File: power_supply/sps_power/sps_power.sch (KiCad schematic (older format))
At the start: 10 parts, among them U1 MC33063AD

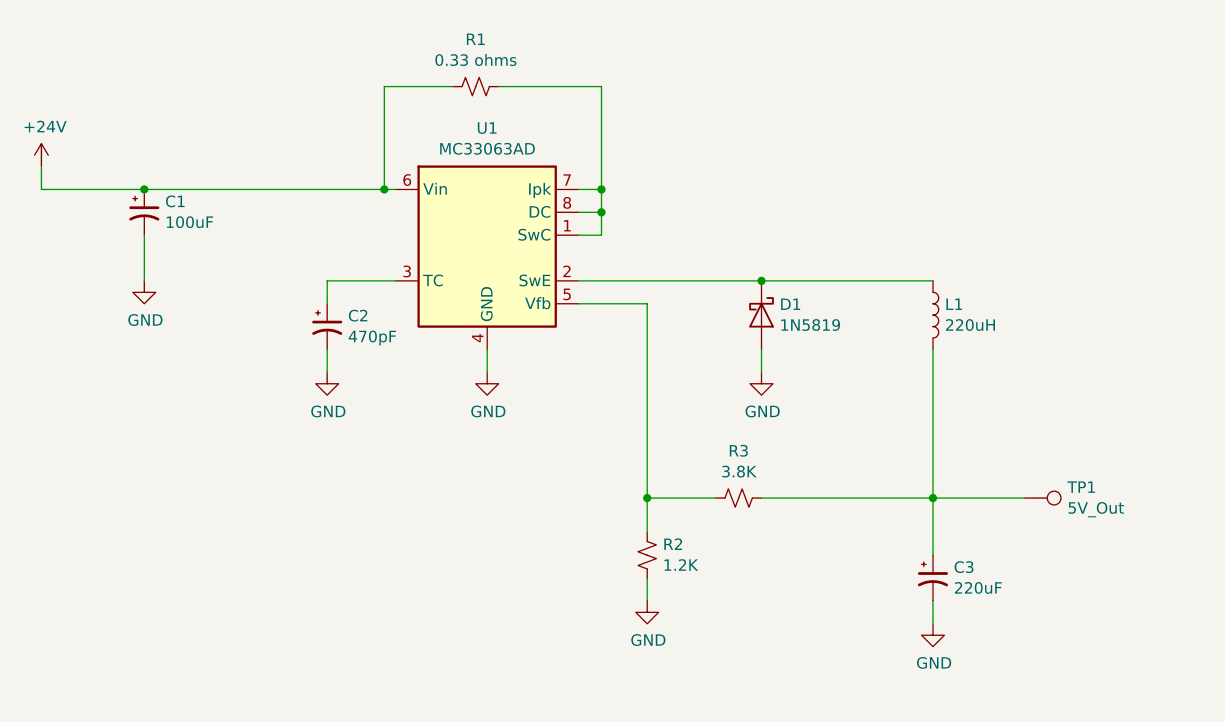
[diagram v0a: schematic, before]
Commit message: Interum power supply cad commit
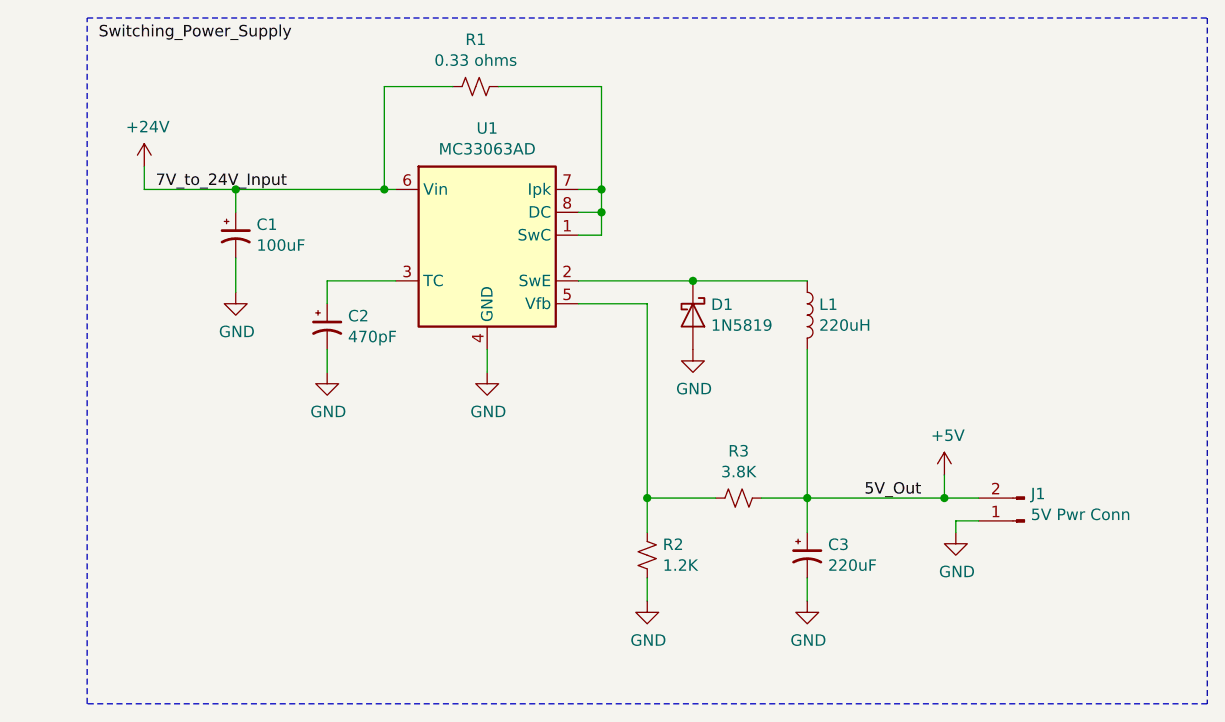
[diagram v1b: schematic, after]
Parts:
- removed TP1: 5V_Out, TestPoint:TestPoint_Pad_D2.0mm, symbol Connector:TestPoint
- added J1: 5V Pwr Conn, Connector_PinHeader_1.00mm:PinHeader_1x02_P1.00mm_Vertical, symbol Connector:Conn_01x02_Male
- U1: Supplier (none) -> DigiKey; Supplier Part (none) -> 296-17763-1-ND
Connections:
- net GND: now also J1.1 (Pin_1)
- net +5V: now reaches C3.1, L1.2, R3.2
- net +5V: now also J1.2 (Pin_2)
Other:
- moved on the sheet: C1, C3, D1, L1
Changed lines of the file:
@@
 $EndDescr
-$Comp
-L Regulator_Switching:MC33063AD U1
-U 1 1 5E7FFA3D
-P 4850 3550
-F 0 "U1" H 4850 4017 50  0000 C CNN
-F 1 "MC33063AD" H 4850 3926 50  0000 C CNN
-F 2 "Package_SO:SOIC-8_3.9x4.9mm_P1.27mm" H 4900 3100 50  0001 L CNN
-F 3 "http://www.onsemi.com/pub_link/Collateral/MC34063A-D.PDF" H 5350 3450 50  0001 C CNN
-	1    4850 3550
-	1    0    0    -1
-$EndComp
 $Comp
 L power:GND #PWR0101
@@
 L Device:CP1_Small C3
 U 1 1 5E805CD8
-P 6800 5050
-F 0 "C3" H 6891 5096 50  0000 L CNN
-F 1 "220uF" H 6891 5005 50  0000 L CNN
-F 2 "Capacitor_SMD:CP_Elec_10x10" H 6800 5050 50  0001 C CNN
-F 3 "~" H 6800 5050 50  0001 C CNN
-F 4 "493-6277-1-ND" H 6800 5050 50  0001 C CNN "Supplier Part"
-F 5 "Digikey" H 6800 5050 50  0001 C CNN "Supplier"
-	1    6800 5050
+P 6250 4950
+F 0 "C3" H 6341 4996 50  0000 L CNN
+F 1 "220uF" H 6341 4905 50  0000 L CNN
+F 2 "Capacitor_SMD:CP_Elec_10x10" H 6250 4950 50  0001 C CNN
+F 3 "~" H 6250 4950 50  0001 C CNN
+F 4 "493-6277-1-ND" H 6250 4950 50  0001 C CNN "Supplier Part"
+F 5 "Digikey" H 6250 4950 50  0001 C CNN "Supplier"
+	1    6250 4950
 	1    0    0    -1
 $EndComp
@@
 L Device:D_Schottky D1
 U 1 1 5E806E01
-P 6050 3900
-F 0 "D1" V 6004 3979 50  0000 L CNN
-F 1 "1N5819" V 6095 3979 50  0000 L CNN
-F 2 "Diode_SMD:D_SOD-123" H 6050 3900 50  0001 C CNN
-F 3 "~" H 6050 3900 50  0001 C CNN
-F 4 "DigiKey" V 6050 3900 50  0001 C CNN "Supplier"
-F 5 "1N5819HW-FDIDKR-ND" V 6050 3900 50  0001 C CNN "Supplier Part"
-	1    6050 3900
+P 5750 3900
+F 0 "D1" V 5704 3979 50  0000 L CNN
+F 1 "1N5819" V 5795 3979 50  0000 L CNN
+F 2 "Diode_SMD:D_SOD-123" H 5750 3900 50  0001 C CNN
+F 3 "~" H 5750 3900 50  0001 C CNN
+F 4 "DigiKey" V 5750 3900 50  0001 C CNN "Supplier"
+F 5 "1N5819HW-FDIDKR-ND" V 5750 3900 50  0001 C CNN "Supplier Part"
+	1    5750 3900
 	0    1    1    0
-$EndComp
-$Comp
-L Device:CP1_Small C1
-U 1 1 5E810EBD
-P 3350 3450
-F 0 "C1" H 3441 3496 50  0000 L CNN
-F 1 "100uF" H 3441 3405 50  0000 L CNN
-F 2 "Capacitor_THT:CP_Radial_D5.0mm_P2.50mm" H 3350 3450 50  0001 C CNN
-F 3 "~" H 3350 3450 50  0001 C CNN
-F 4 "493-2203-1-ND" H 3350 3450 50  0001 C CNN "Supplier Part"
-F 5 "Digikey" H 3350 3450 50  0001 C CNN "Supplier"
-	1    3350 3450
-	1    0    0    -1
 $EndComp
 $Comp
 L power:GND #PWR0103
 U 1 1 5E81AA34
-P 3350 3750
-F 0 "#PWR0103" H 3350 3500 50  0001 C CNN
-F 1 "GND" H 3355 3577 50  0000 C CNN
-F 2 "" H 3350 3750 50  0001 C CNN
-F 3 "" H 3350 3750 50  0001 C CNN
-	1    3350 3750
-	1    0    0    -1
-$EndComp
-Wire Wire Line
-	3350 3550 3350 3750
+P 3750 3800
+F 0 "#PWR0103" H 3750 3550 50  0001 C CNN
+F 1 "GND" H 3755 3627 50  0000 C CNN
+F 2 "" H 3750 3800 50  0001 C CNN
+F 3 "" H 3750 3800 50  0001 C CNN
+	1    3750 3800
+	1    0    0    -1
+$EndComp
 $Comp
 L Device:R_Small_US R3
@@
 	5250 3350 5350 3350
 Wire Wire Line
-	2900 3250 2900 3350
-Wire Wire Line
-	2900 3350 3350 3350
-Connection ~ 3350 3350
-Wire Wire Line
-	3350 3350 4400 3350
-Wire Wire Line
 	4450 3350 4400 3350
 Connection ~ 4400 3350
@@
 Connection ~ 5350 3450
 Wire Wire Line
-	5250 3750 6050 3750
+	5250 3750 5750 3750
 $Comp
 L Device:L L1
 U 1 1 5E801D9A
-P 6800 3900
-F 0 "L1" H 6852 3946 50  0000 L CNN
-F 1 "220uH" H 6852 3855 50  0000 L CNN
-F 2 "Inductor_SMD:L_Bourns-SRR1005" H 6800 3900 50  0001 C CNN
-F 3 "~" H 6800 3900 50  0001 C CNN
-F 4 "Digikey" H 6800 3900 50  0001 C CNN "Supplier"
-F 5 "SDR1806-221KLCT-ND" H 6800 3900 50  0001 C CNN "Supplier Part"
-	1    6800 3900
-	1    0    0    -1
-$EndComp
-Wire Wire Line
-	6050 3750 6800 3750
-Connection ~ 6050 3750
+P 6250 3900
+F 0 "L1" H 6302 3946 50  0000 L CNN
+F 1 "220uH" H 6302 3855 50  0000 L CNN
+F 2 "Inductor_SMD:L_Bourns-SRR1005" H 6250 3900 50  0001 C CNN
+F 3 "~" H 6250 3900 50  0001 C CNN
+F 4 "Digikey" H 6250 3900 50  0001 C CNN "Supplier"
+F 5 "SDR1806-221KLCT-ND" H 6250 3900 50  0001 C CNN "Supplier Part"
+	1    6250 3900
+	1    0    0    -1
+$EndComp
 Wire Wire Line
 	4850 4050 4850 4150
@@
 L power:GND #PWR0105
 U 1 1 5E863A3A
-P 6800 5250
-F 0 "#PWR0105" H 6800 5000 50  0001 C CNN
-F 1 "GND" H 6805 5077 50  0000 C CNN
-F 2 "" H 6800 5250 50  0001 C CNN
-F 3 "" H 6800 5250 50  0001 C CNN
-	1    6800 5250
-	1    0    0    -1
-$EndComp
-Wire Wire Line
-	6800 5150 6800 5250
-Wire Wire Line
-	6800 4050 6800 4700
+P 6250 5150
+F 0 "#PWR0105" H 6250 4900 50  0001 C CNN
+F 1 "GND" H 6255 4977 50  0000 C CNN
+F 2 "" H 6250 5150 50  0001 C CNN
+F 3 "" H 6250 5150 50  0001 C CNN
+	1    6250 5150
+	1    0    0    -1
+$EndComp
 Wire Wire Line
 	5250 3850 5550 3850
@@
 Connection ~ 5550 4700
 Wire Wire Line
-	6050 4700 6800 4700
-Connection ~ 6800 4700
-Wire Wire Line
-	6800 4700 6800 4950
-$Comp
-L Connector:TestPoint TP1
-U 1 1 5E86A93E
-P 7200 4700
-F 0 "TP1" V 7154 4888 50  0000 L CNN
-F 1 "5V_Out" V 7245 4888 50  0000 L CNN
-F 2 "TestPoint:TestPoint_Pad_D2.0mm" H 7400 4700 50  0001 C CNN
-F 3 "~" H 7400 4700 50  0001 C CNN
-	1    7200 4700
-	0    1    1    0
-$EndComp
-Wire Wire Line
-	6800 4700 7200 4700
+	6050 4700 6250 4700
 $Comp
 L power:GND #PWR0106
 U 1 1 5E86CC9B
-P 6050 4150
-F 0 "#PWR0106" H 6050 3900 50  0001 C CNN
-F 1 "GND" H 6055 3977 50  0000 C CNN
-F 2 "" H 6050 4150 50  0001 C CNN
-F 3 "" H 6050 4150 50  0001 C CNN
-	1    6050 4150
-	1    0    0    -1
-$EndComp
-Wire Wire Line
-	6050 4050 6050 4150
+P 5750 4050
+F 0 "#PWR0106" H 5750 3800 50  0001 C CNN
+F 1 "GND" H 5755 3877 50  0000 C CNN
+F 2 "" H 5750 4050 50  0001 C CNN
+F 3 "" H 5750 4050 50  0001 C CNN
+	1    5750 4050
+	1    0    0    -1
+$EndComp
 $Comp
 L Device:CP1_Small C2
@@
 L power:+24V #PWR0102
 U 1 1 5E820AB8
-P 2900 3250
-F 0 "#PWR0102" H 2900 3100 50  0001 C CNN
-F 1 "+24V" H 2915 3423 50  0000 C CNN
-F 2 "" H 2900 3250 50  0001 C CNN
-F 3 "" H 2900 3250 50  0001 C CNN
-	1    2900 3250
-	1    0    0    -1
-$EndComp
+P 3350 3250
+F 0 "#PWR0102" H 3350 3100 50  0001 C CNN
+F 1 "+24V" H 3365 3423 50  0000 C CNN
+F 2 "" H 3350 3250 50  0001 C CNN
+F 3 "" H 3350 3250 50  0001 C CNN
+	1    3350 3250
+	1    0    0    -1
+$EndComp
+Connection ~ 5750 3750
+Wire Wire Line
+	5750 3750 6250 3750
+Wire Wire Line
+	6250 4050 6250 4700
+Connection ~ 6250 4700
+Wire Wire Line
+	6250 4700 6250 4850
+Wire Wire Line
+	6250 5050 6250 5150
+$Comp
+L Connector:Conn_01x02_Male J1
+U 1 1 5E86AA57
+P 7200 4800
+F 0 "J1" H 7172 4682 50  0000 R CNN
+F 1 "5V Pwr Conn" H 7172 4773 50  0000 R CNN
+F 2 "Connector_PinHeader_1.00mm:PinHeader_1x02_P1.00mm_Vertical" H 7200 4800 50  0001 C CNN
+F 3 "~" H 7200 4800 50  0001 C CNN
+	1    7200 4800
+	-1   0    0    1
+$EndComp
+$Comp
+L power:GND #PWR0108
+U 1 1 5E86FA5C
+P 6900 4850
+F 0 "#PWR0108" H 6900 4600 50  0001 C CNN
+F 1 "GND" H 6905 4677 50  0000 C CNN
+F 2 "" H 6900 4850 50  0001 C CNN
+F 3 "" H 6900 4850 50  0001 C CNN
+	1    6900 4850
+	1    0    0    -1
+$EndComp
+$Comp
+L Regulator_Switching:MC33063AD U1
+U 1 1 5E7FFA3D
+P 4850 3550
+F 0 "U1" H 4850 4017 50  0000 C CNN
+F 1 "MC33063AD" H 4850 3926 50  0000 C CNN
+F 2 "Package_SO:SOIC-8_3.9x4.9mm_P1.27mm" H 4900 3100 50  0001 L CNN
+F 3 "http://www.onsemi.com/pub_link/Collateral/MC34063A-D.PDF" H 5350 3450 50  0001 C CNN
+F 4 "DigiKey" H 4850 3550 50  0001 C CNN "Supplier"
+F 5 "296-17763-1-ND" H 4850 3550 50  0001 C CNN "Supplier Part"
+	1    4850 3550
+	1    0    0    -1
+$EndComp
+Wire Wire Line
+	3350 3250 3350 3350
+Wire Notes Line style solid
+	3100 2600 8000 2600
+Wire Notes Line style solid
+	8000 2600 8000 5600
+Wire Notes Line style solid
+	8000 5600 3100 5600
+Wire Notes Line style solid
+	3100 5600 3100 2600
+Text Label 6500 4700 0    50   ~ 0
+5V_Out
+Text Label 3400 3350 0    50   ~ 0
+7V_to_24V_Input
+Text Label 3150 2700 0    50   ~ 0
+Switching_Power_Supply
+Wire Wire Line
+	6250 4700 6850 4700
+Wire Wire Line
+	6900 4850 6900 4800
+Wire Wire Line
+	6900 4800 7000 4800
+$Comp
+L Device:CP1_Small C1
+U 1 1 5E810EBD
+P 3750 3550
+F 0 "C1" H 3841 3596 50  0000 L CNN
+F 1 "100uF" H 3841 3505 50  0000 L CNN
+F 2 "Capacitor_THT:CP_Radial_D5.0mm_P2.50mm" H 3750 3550 50  0001 C CNN
+F 3 "~" H 3750 3550 50  0001 C CNN
+F 4 "493-2203-1-ND" H 3750 3550 50  0001 C CNN "Supplier Part"
+F 5 "Digikey" H 3750 3550 50  0001 C CNN "Supplier"
+	1    3750 3550
+	1    0    0    -1
+$EndComp
+Wire Wire Line
+	3350 3350 3750 3350
+Wire Wire Line
+	3750 3450 3750 3350
+Connection ~ 3750 3350
+Wire Wire Line
+	3750 3350 4400 3350
+Wire Wire Line
+	3750 3650 3750 3800
+$Comp
+L power:+5V #PWR?
+U 1 1 5E84131D
+P 6850 4600
+F 0 "#PWR?" H 6850 4450 50  0001 C CNN
+F 1 "+5V" H 6865 4773 50  0000 C CNN
+F 2 "" H 6850 4600 50  0001 C CNN
+F 3 "" H 6850 4600 50  0001 C CNN
+	1    6850 4600
+	1    0    0    -1
+$EndComp
+Wire Wire Line
+	6850 4600 6850 4700
+Connection ~ 6850 4700
+Wire Wire Line
+	6850 4700 7000 4700
 $EndSCHEMATC

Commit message: Copied power supply circuit into signal board schematic, initial creation of PCB
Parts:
- D1: Supplier Part 1N5819HW-FDIDKR-ND -> 1N5819HW-FDICT-ND
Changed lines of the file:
@@
 F 3 "~" H 5750 3900 50  0001 C CNN
 F 4 "DigiKey" V 5750 3900 50  0001 C CNN "Supplier"
-F 5 "1N5819HW-FDIDKR-ND" V 5750 3900 50  0001 C CNN "Supplier Part"
+F 5 "1N5819HW-FDICT-ND" V 5750 3900 50  0001 C CNN "Supplier Part"
 	1    5750 3900
 	0    1    1    0
